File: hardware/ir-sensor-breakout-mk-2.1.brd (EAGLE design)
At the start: 24 x 29 mm, 6 parts, among them U1 MLX906145V-PTH

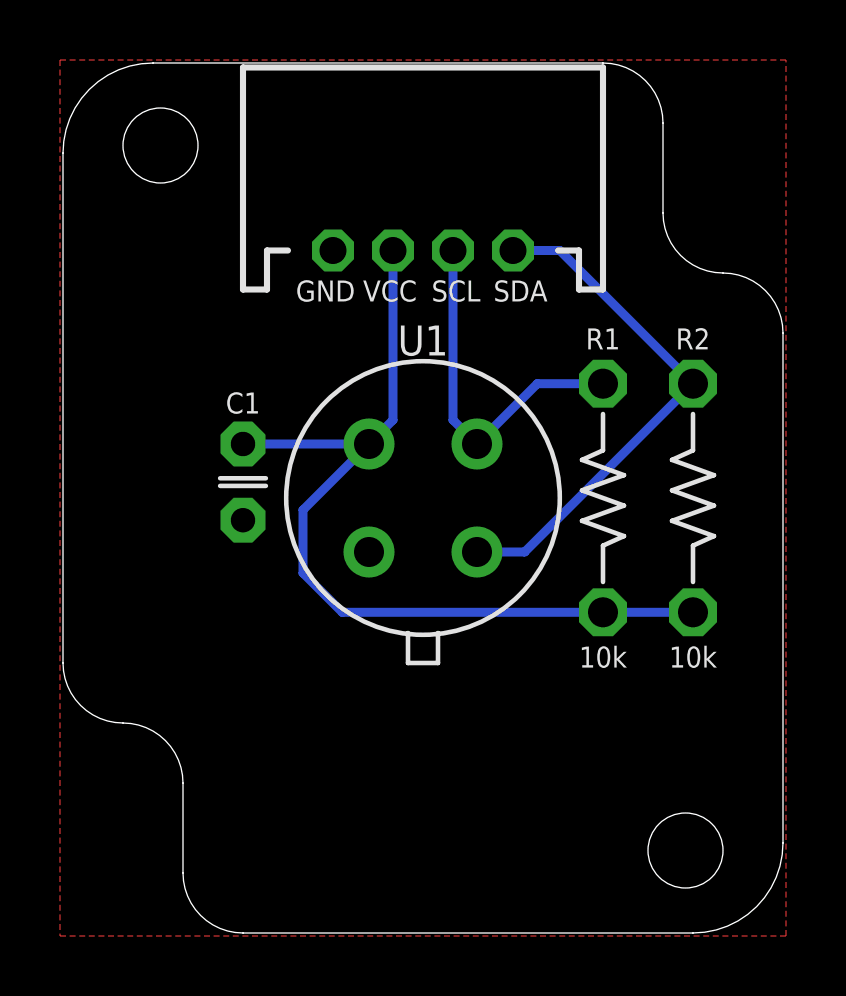
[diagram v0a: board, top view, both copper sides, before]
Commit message: twiddling around with IR sensor breakouts
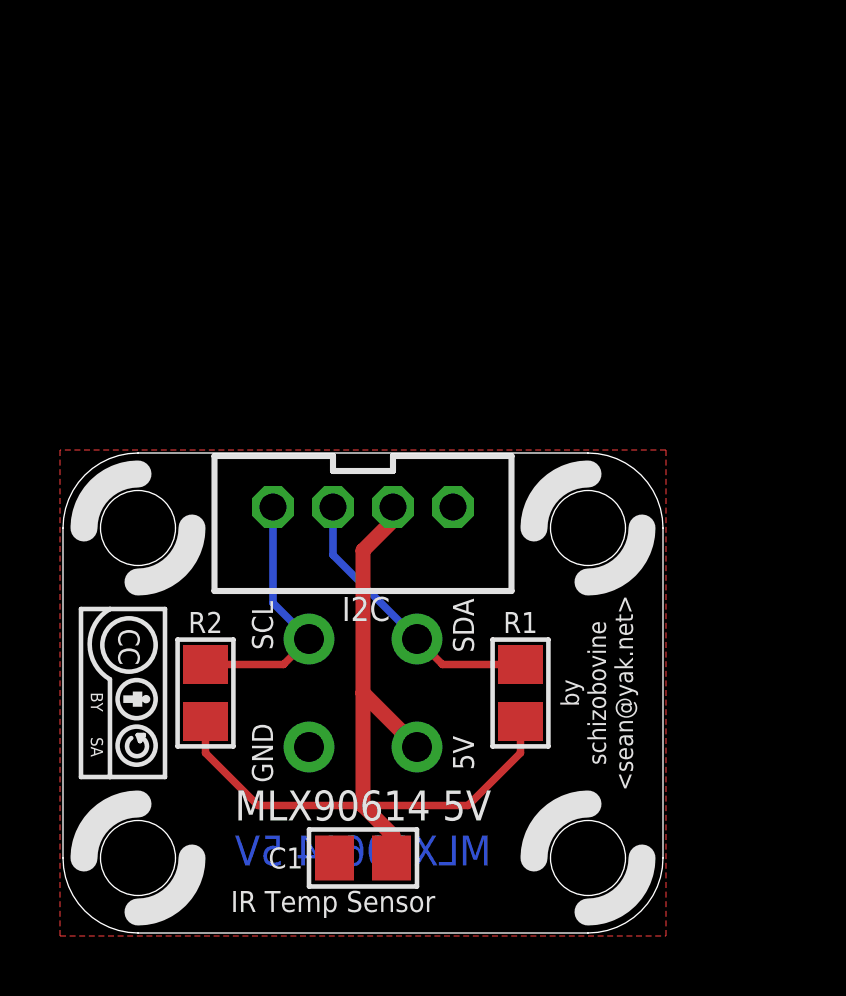
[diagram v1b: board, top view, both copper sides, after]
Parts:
- removed JP1: M04JST-PTH, A_butts:JST-4-PH-RA-PTH
- added H1, H2, H3, H4: HOLE#2, A_butts:HOLE-#2
- added I2C: M04JST-PTH-VERT, A_butts:JST-4-PH-VERT-PTH
- added U$1: CC-BY-SA-4.0NO-URL, A_butts:CC-BY-SA-4.0-NO-URL
- C1: value 0.1uF -> 100nF; device A_butts:C025-024X044 -> A_butts:C0805
- FRAME1: value (none) -> FRAME-LETTERNO_PACKAGE
- R1, R2: device A_butts:RESISTOR-AXIAL-PTH-7.62MM -> A_butts:R0805
- moved R2 17.5 mm to (4.75, 8.00)
- moved C1 13.2 mm to (10.0, 2.50), turned to 180 degrees
- moved R1 7.06 mm to (15.2, 8.00)
- moved U1 6.80 mm to (10.0, 8.00), flipped to the bottom, turned to 270 degrees
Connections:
- net GND: now also I2C.1; no longer JP1.1
- net SCL: now also I2C.4, R2.1; no longer JP1.4, R2.P$1
- net SDA: now also I2C.3, R1.1; no longer JP1.3, R1.P$1
- net VCC: now also I2C.2, R1.2, R2.2; no longer JP1.2, R1.P$2, R2.P$2
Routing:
- net SCL: track 17.4 -> 8.70 mm
- net SDA: track 11.8 -> 9.36 mm
- net VCC: track 29.7 -> 29.1 mm
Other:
- board size 24 x 29 mm -> 20 x 16 mm
- board text added: "5V"
- board text added: ">VERSION"
- board text added: "IR Temp Sensor"
- board text added: "MLX90614 5V"
- board text added: "by schizobovine <sean@yak.net>"
- board text removed: "VCC"
